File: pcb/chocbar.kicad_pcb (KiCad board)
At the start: 2 copper layers, 211.2 x 87.5 mm, 132 parts, among them SW1 SW_PUSH, SW10 SW_PUSH, SW11 SW_PUSH, SW12 SW_PUSH, SW13 SW_PUSH, SW14 SW_PUSH, SW15 SW_PUSH, SW16 SW_PUSH, SW17 SW_PUSH, SW18 SW_PUSH, SW19 SW_PUSH, SW2 SW_PUSH, SW20 SW_PUSH, SW21 SW_PUSH, SW22 SW_PUSH, SW23 SW_PUSH, SW24 SW_PUSH, SW25 SW_PUSH, SW26 SW_PUSH, SW27 SW_PUSH, SW28 SW_PUSH, SW29 SW_PUSH, SW3 SW_PUSH, SW30 SW_PUSH, SW31 SW_PUSH, SW32 SW_PUSH, SW33 SW_PUSH, SW34 SW_PUSH, SW35 SW_PUSH, SW36 SW_PUSH, SW37 SW_PUSH, SW38 SW_PUSH, SW39 SW_PUSH, SW4 SW_PUSH, SW40 SW_PUSH, SW41 SW_PUSH, SW42 SW_PUSH, SW5 SW_PUSH, SW6 SW_PUSH, SW7 SW_PUSH, SW8 SW_PUSH, SW9 SW_PUSH, U1 ProMicro

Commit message: improve
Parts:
- removed D41, D42: D, mikamo3:D3_SMD_1side
- removed HOLE_1, HOLE_2, HOLE_3: Val**, foostan:M2_HOLE_v2
- removed L41, L42: SK6812MINI-E, swanmatch:YS-SK6812MINI-E
- removed SW41, SW42: SW_PUSH, mikamo3:Choc_Hotswap_1side
- added H1: Val**, foostan:M2_HOLE_v2, F.Cu at (57.2, 113.6)
- added H2: Val**, foostan:M2_HOLE_v2, F.Cu at (75.2, 113.6)
- added H3: Val**, foostan:M2_HOLE_v2, F.Cu at (116.7, 121.5)
- added H4: Val**, foostan:M2_HOLE_v2, F.Cu at (173.8, 121.5)
- added H5: Val**, foostan:M2_HOLE_v2, F.Cu at (231.0, 121.5)
- OL1: footprint foostan:OLED_1side -> mikamo3:OLED_1side
- SW33, SW34, SW35, SW36: footprint mikamo3:Choc_Hotswap_1side -> mikamo3:Choc_Hotswap_1.5u_1side
- moved L40 171.2 mm to (69.1, 145.3)
- moved SW40 171.1 mm to (69.1, 150.0)
- moved D40 170.0 mm to (76.2, 154.2)
- moved D39 148.9 mm to (76.2, 135.1)
- moved L39 147.9 mm to (69.1, 126.3)
- moved SW39 147.8 mm to (69.1, 131.0)
- moved SW_RESET1 93.5 mm to (65.8, 118.8), turned to 180 degrees
- moved L37 82.6 mm to (240.5, 145.3)
- moved L38 82.6 mm to (259.6, 145.3)
- moved SW37 82.4 mm to (240.5, 150.0)
- moved SW38 82.4 mm to (259.6, 150.0)
- moved D37 81.6 mm to (247.7, 154.2)
- moved D38 81.6 mm to (266.7, 154.2)
- moved L36 78.9 mm to (216.7, 145.3)
- moved SW36 78.7 mm to (216.7, 150.0)
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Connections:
- D10 pad 1: row1 -> row0
- D15 pad 1: row2 -> row1
- D16 pad 1: row2 -> row1
- D17 pad 1: row2 -> row1
- D18 pad 1: row2 -> row1
- D19 pad 1: row2 -> row1
- D20 pad 1: row2 -> row1
- D22 pad 1: row3 -> row2
- D23 pad 1: row3 -> row2
- D24 pad 1: row3 -> row2
- D25 pad 1: row3 -> row2
- D26 pad 1: row3 -> row2
- D27 pad 1: row3 -> row2
- D28 pad 1: row3 -> row2
- D29 pad 1: row4 -> row2
- D30 pad 1: row4 -> row2
- D31 pad 1: row4 -> row3
- D32 pad 1: row4 -> row3
- D33 pad 1: row4 -> row3
- D34 pad 1: row4 -> row3
- D35 pad 1: row4 -> row3
- D36 pad 1: row5 -> row3
- D37 pad 1: row5 -> row3
- D38 pad 1: row5 -> row3
- D39 pad 1: row5 -> row3
- D40 pad 1: row5 -> row3
- D8 pad 1: row1 -> row0
- D9 pad 1: row1 -> row0
- L40 pad 2: Net-(L40-Pad2) -> (no net)
- SW10 pad 1: col2 -> col9
- SW11 pad 1: col3 -> col0
- SW12 pad 1: col4 -> col1
- SW13 pad 1: col5 -> col2
- SW14 pad 1: col6 -> col3
- SW15 pad 1: col0 -> col4
- SW16 pad 1: col1 -> col5
- SW17 pad 1: col2 -> col6
- SW18 pad 1: col3 -> col7
- SW19 pad 1: col4 -> col8
- SW20 pad 1: col5 -> col9
- SW21 pad 1: col6 -> col0
- SW22 pad 1: col0 -> col1
- SW23 pad 1: col1 -> col2
- SW24 pad 1: col2 -> col3
- SW25 pad 1: col3 -> col4
- SW26 pad 1: col4 -> col5
- SW27 pad 1: col5 -> col6
- SW28 pad 1: col6 -> col7
- SW29 pad 1: col0 -> col8
- SW30 pad 1: col1 -> col9
- SW31 pad 1: col2 -> col0
- SW32 pad 1: col3 -> col1
- SW33 pad 1: col4 -> col2
- SW34 pad 1: col5 -> col3
- SW35 pad 1: col6 -> col4
- SW36 pad 1: col0 -> col5
- SW37 pad 1: col1 -> col6
- SW38 pad 1: col2 -> col7
- SW39 pad 1: col3 -> col8
- SW40 pad 1: col4 -> col9
- SW8 pad 1: col0 -> col7
- SW9 pad 1: col1 -> col8
- U1 pad 11: row4 -> col0
- U1 pad 12: row5 -> col1
- U1 pad 13: (no net) -> col9
- U1 pad 14: col6 -> col8
- U1 pad 15: col5 -> col7
- U1 pad 16: col4 -> col6
- U1 pad 17: col3 -> col5
- U1 pad 18: col2 -> col4
- U1 pad 19: col1 -> col3
- U1 pad 20: col0 -> col2
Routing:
- net col7: track 0.00 -> 356.6 mm, vias 0 -> 7
- net col8: track 0.00 -> 348.2 mm, vias 0 -> 7
- net col9: track 0.00 -> 323.9 mm, vias 0 -> 6
- net col0: track 400.3 -> 84.8 mm, vias 7 -> 4
- net col1: track 437.0 -> 144.1 mm, vias 8 -> 5
- net row4: track 260.4 -> 0.00 mm, vias 2 -> 0
- net Net-(L38-Pad2): track 15.3 -> 267.3 mm
- net row5: track 251.3 -> 0.00 mm
- net Net-(L40-Pad2): track 209.5 -> 0.00 mm, vias 2 -> 0
- net col2: track 480.9 -> 286.6 mm, vias 6 -> 8
- net col4: track 410.0 -> 308.0 mm, vias 7 -> 10
- net row3: track 194.4 -> 280.2 mm, vias 5 -> 3
- net GND: track 1024.4 -> 941.5 mm, vias 42 -> 40
- net Net-(L41-Pad2): track 55.8 -> 0.00 mm, vias 2 -> 0
- net col5: track 364.4 -> 416.8 mm, vias 5 -> 8
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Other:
- board size 211.2 x 87.5 mm -> 214.2 x 83.1 mm
- board text added: "chocbar v1.0 PCB designed by kamo"

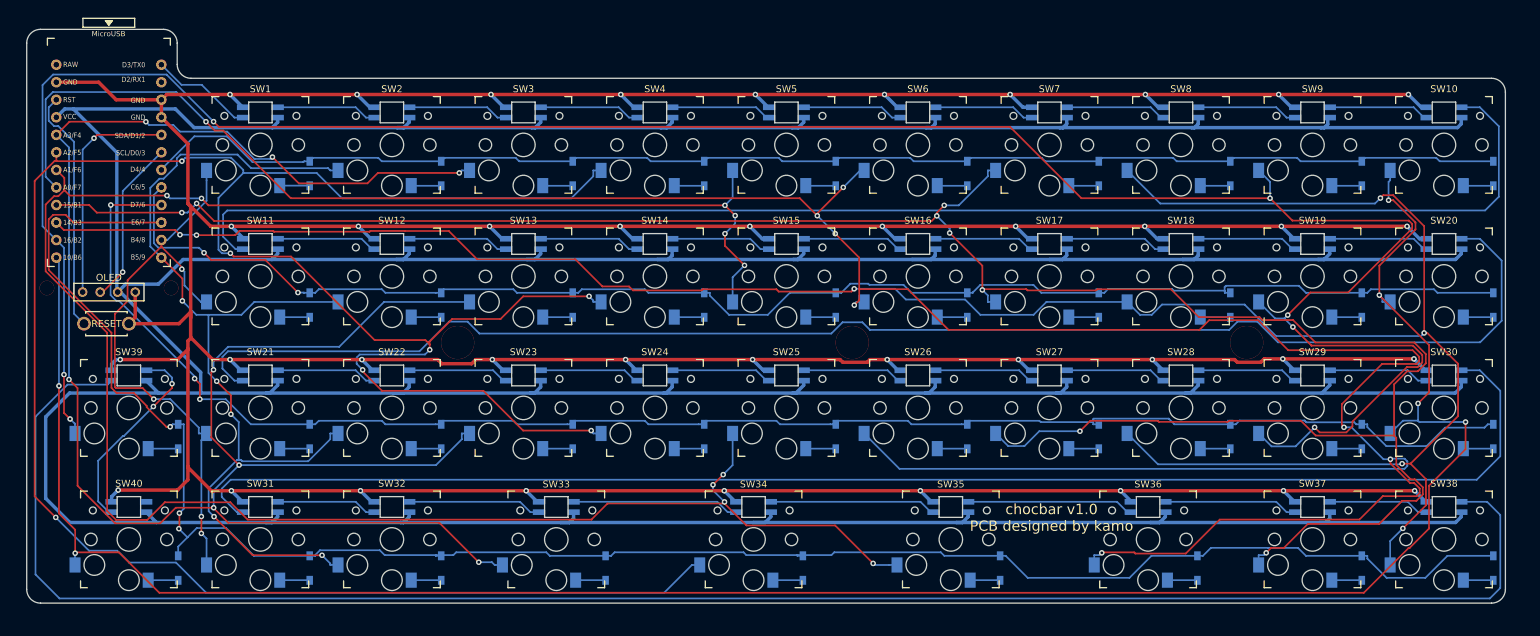
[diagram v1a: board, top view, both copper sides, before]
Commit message: fix pcb and plate
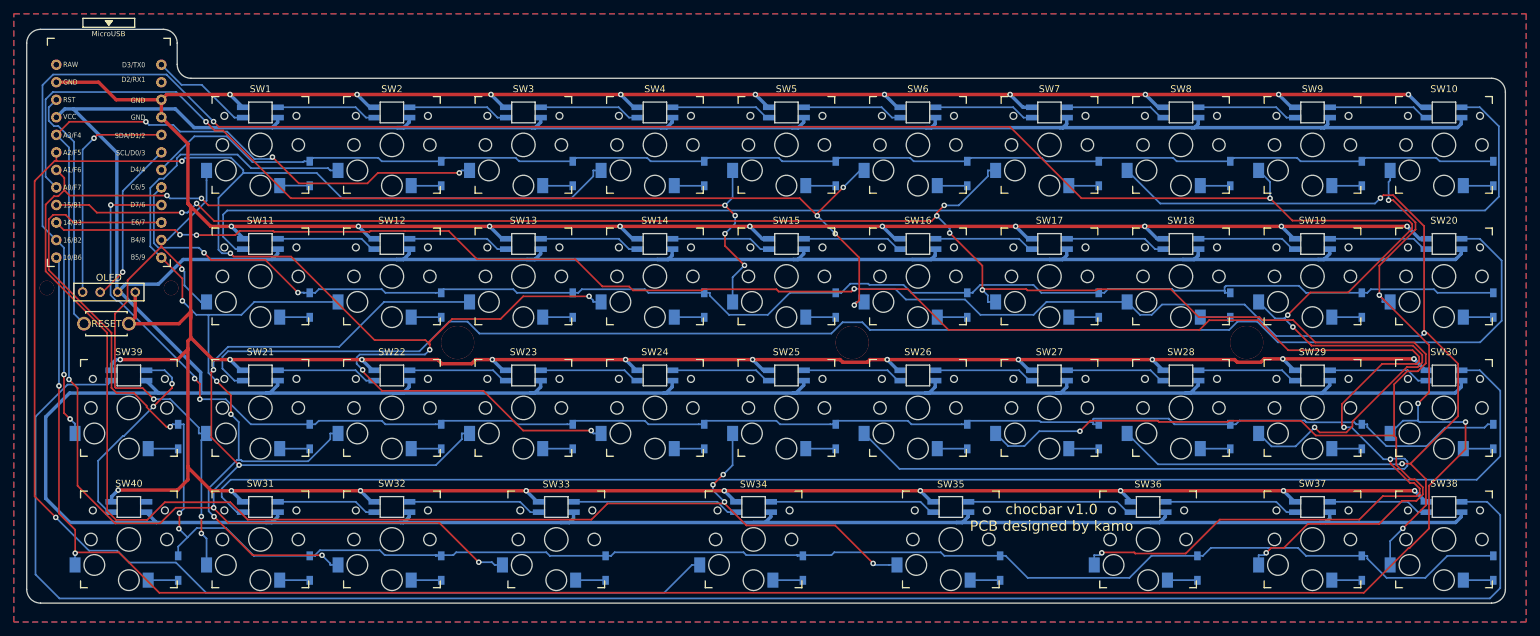
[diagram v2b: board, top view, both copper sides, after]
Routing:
- added copper zone on B.Cu, net GND
- added copper zone on F.Cu, net GND
